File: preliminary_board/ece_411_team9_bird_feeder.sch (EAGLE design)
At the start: 11 parts, among them IC1 TINY13V-10PU, IC2 LM741P, IC3 LM741P, M1 ELECTRET_MICROPHON-WM.64PN, M2 SERVO

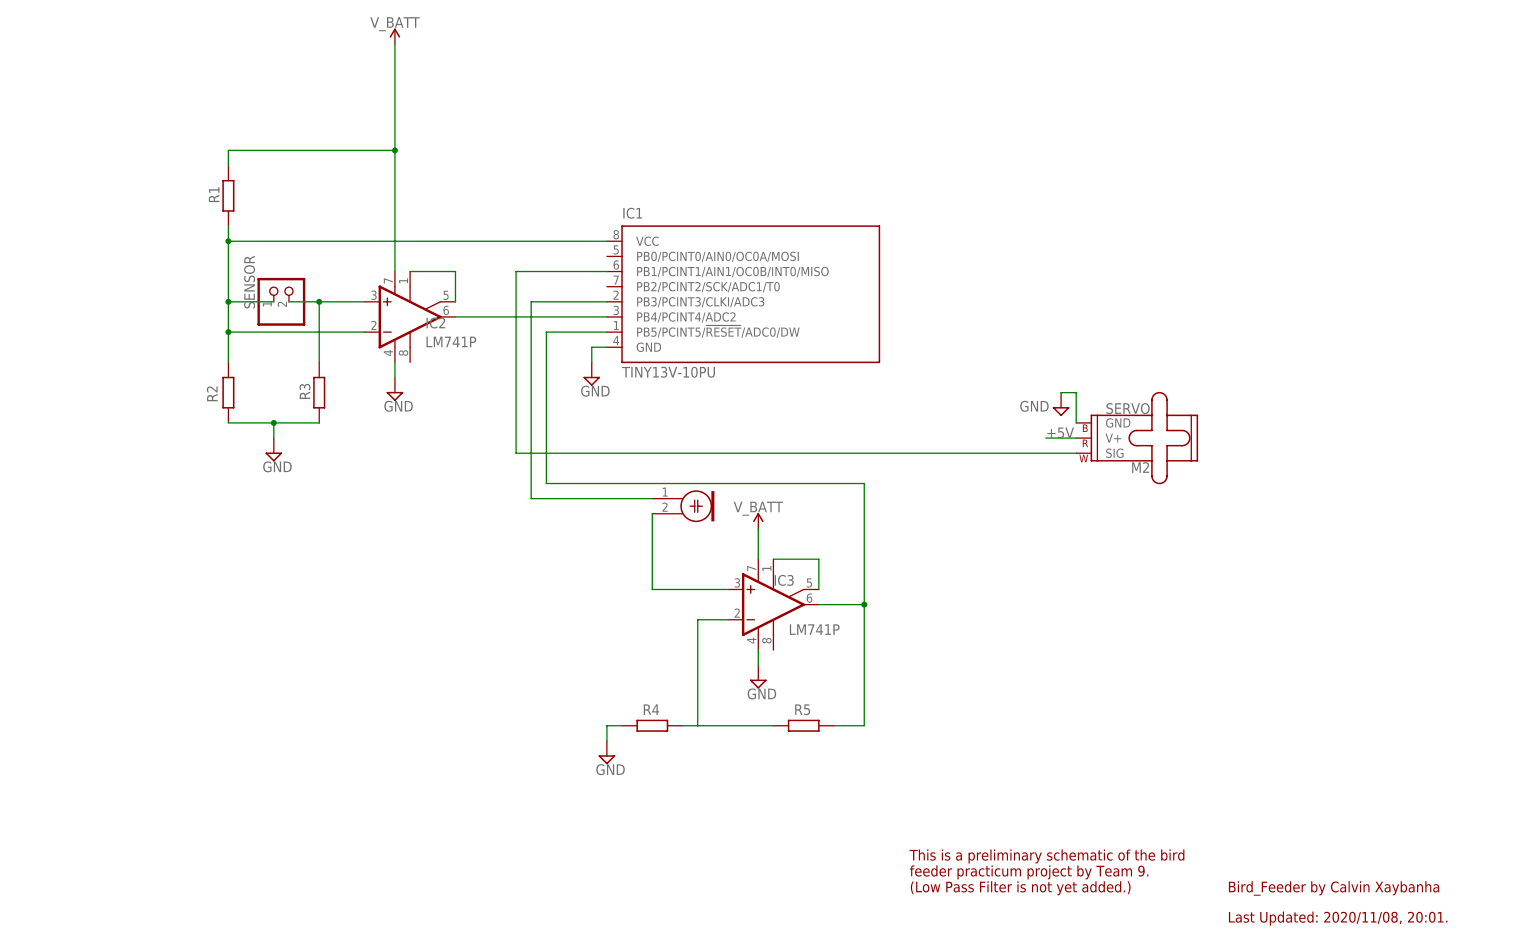
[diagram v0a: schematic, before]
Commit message: Add files via upload
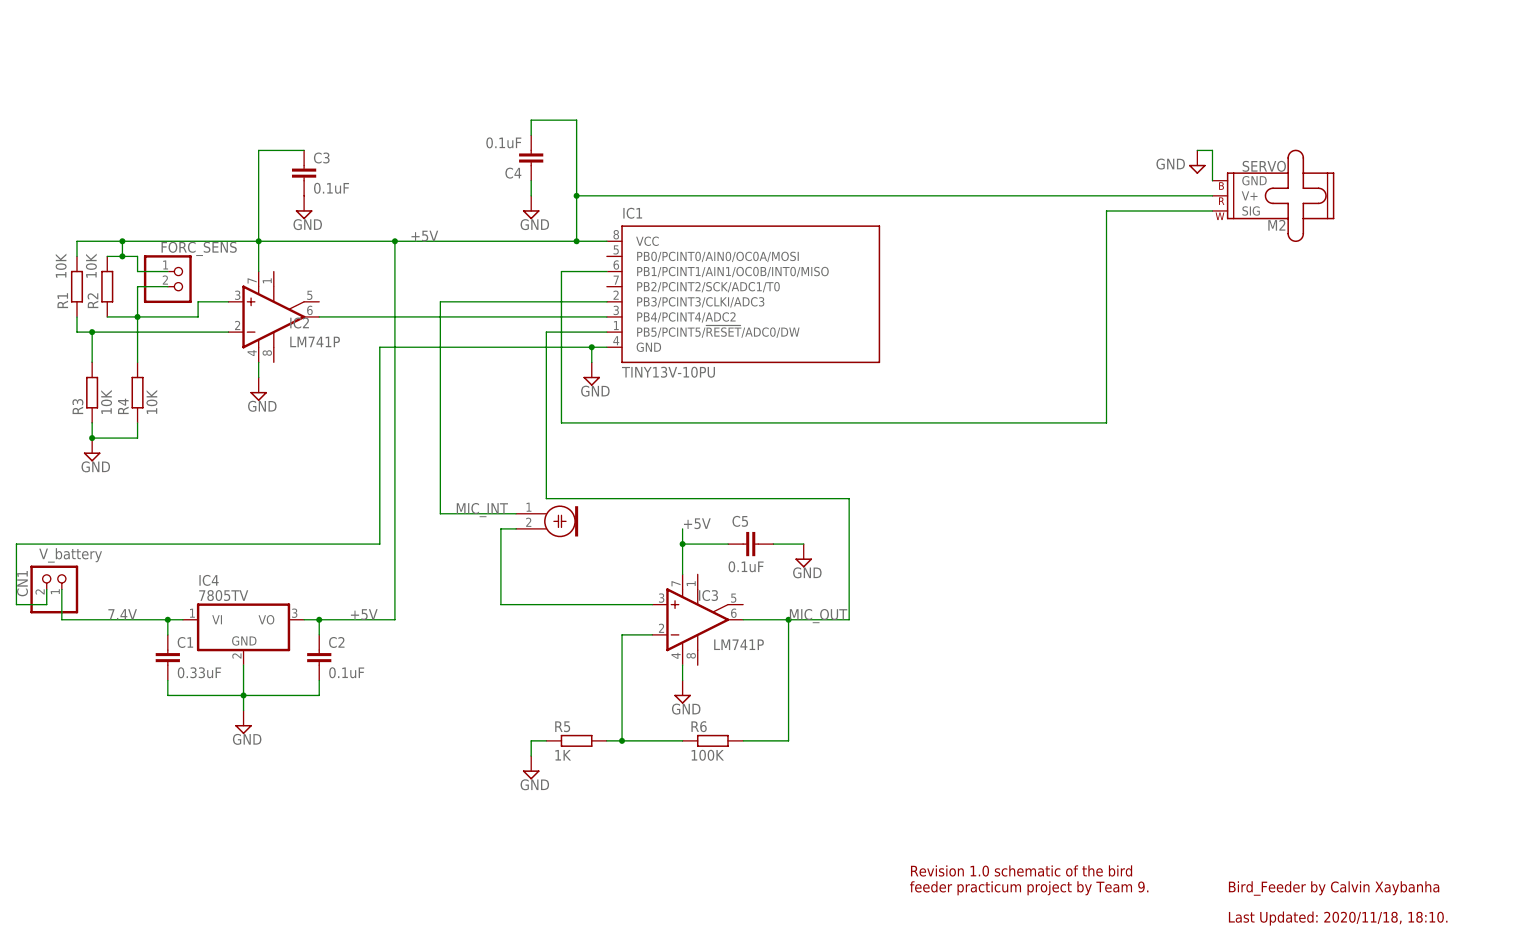
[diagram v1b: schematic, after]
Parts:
- removed SENSOR: (no value), pinhead:PINHD-1X2/90
- added C1: 0.33uF, eagle-ltspice:C
- added C2, C3, C4, C5: 0.1uF, eagle-ltspice:C
- added CN1: V_battery, adafruit:JST_2PIN-SMT
- added FORC_SENS: (no value), pinhead:PINHD-1X2/90
- added IC4: 7805TV, linear:7805TV
- added R6: 100K, eagle-ltspice:R
- R1, R2, R3, R4: value (none) -> 10K; device eagle-ltspice:R0207/10 -> eagle-ltspice:R
- R5: value (none) -> 1K; device eagle-ltspice:R0207/10 -> eagle-ltspice:R
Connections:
- net N$5 renamed MIC_INT
- removed net N$1: IC1.VCC, IC2.-IN, R1.1, R2.1, SENSOR.1
- removed net N$12: IC1.PB5/PCINT5/!RESET!/ADC0/DW, IC3.OUT, R5.1
- removed net N$2: IC2.ON1, IC2.ON2
- removed net N$3: IC3.ON1, IC3.ON2
- removed net V_BATT: IC2.V+, IC3.V+, R1.2
- new net 7.4V: C1.1, CN1.2, IC4.VI
- new net MIC_OUT: IC1.PB5/PCINT5/!RESET!/ADC0/DW, IC3.OUT, R6.2
- new net N$8: IC2.-IN, R1.1, R3.2
- net +5V: now also C2.1, C3.1, C4.2, C5.1, FORC_SENS.1, IC1.VCC, IC2.V+, IC3.V+, IC4.VO, R1.2, R2.2
- net GND: now also C1.2, C2.2, C3.2, C4.1, C5.2, CN1.1, IC4.GND, R4.1, R5.1; no longer R2.2, R4.2
- net N$13: now also R6.1; no longer R4.1
- net N$4: now also FORC_SENS.2, R2.1, R4.2; no longer R3.2, SENSOR.2
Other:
- note added: "Controller"
- note added: "Last Updated: 2020/11/18, 18:10."
- note added: "Revision 1.0 schematic of the bird feeder practicum project by Team 9."
- note added: "Voltage Supply Regular"
- note removed: "Last Updated: 2020/11/08, 20:01."
- note removed: "This is a preliminary schematic of the bird feeder practicum project by Team 9. (Low Pass Filter is not yet added.)"
- moved on the sheet: IC2, IC3, M2, R1, R2, R3, R4, R5
